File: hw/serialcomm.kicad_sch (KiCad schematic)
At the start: 4 parts, among them J2 USB_B_Micro, U17 W65C51NxP, U19 FT232RL, X4 1.8432 MHz

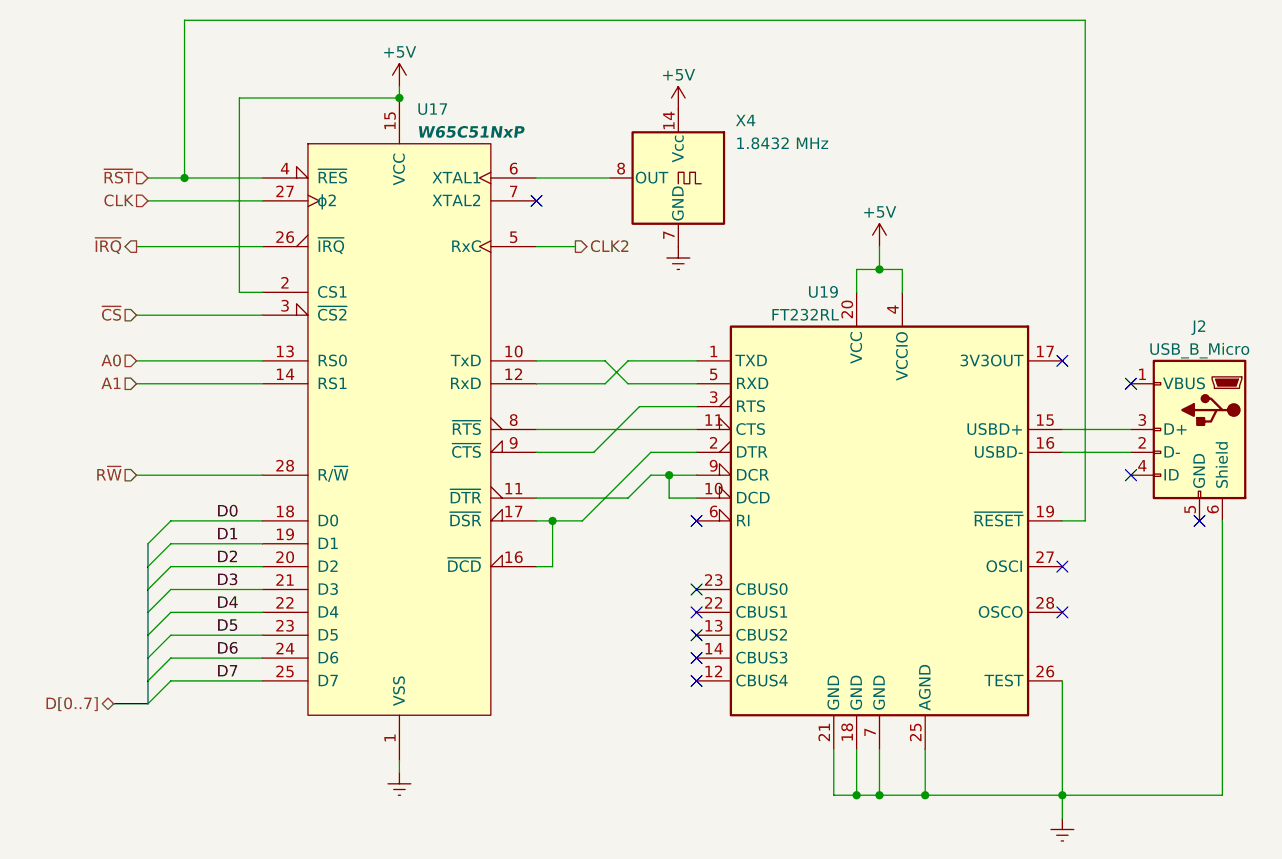
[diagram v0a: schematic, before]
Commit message: add hw design for veraduino
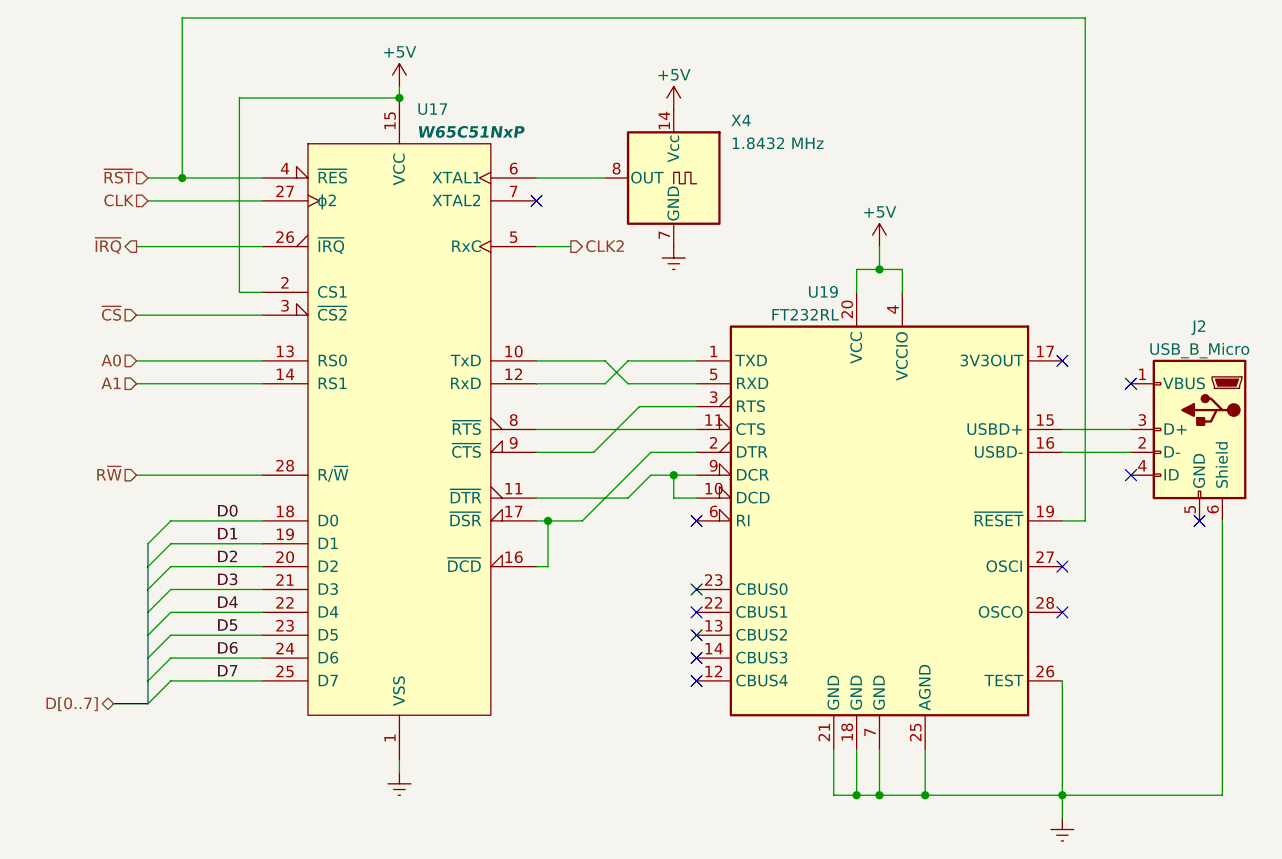
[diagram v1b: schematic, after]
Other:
- moved on the sheet: X4
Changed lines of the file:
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@@
   (junction (at 119.38 106.68) (diameter 0) (color 0 0 0 0)
   )
-  (junction (at 77.978 76.2) (diameter 0) (color 0 0 0 0)
-  )
-  (junction (at 90.932 71.12) (diameter 0) (color 0 0 0 0)
+  (junction (at 77.47 76.2) (diameter 0) (color 0 0 0 0)
+  )
+  (junction (at 91.44 71.12) (diameter 0) (color 0 0 0 0)
   )
   (junction (at 134.62 106.68) (diameter 0) (color 0 0 0 0)
   )
-  (junction (at 37.084 38.1) (diameter 0) (color 0 0 0 0)
+  (junction (at 36.83 38.1) (diameter 0) (color 0 0 0 0)
   )
   (junction (at 114.3 106.68) (diameter 0) (color 0 0 0 0)
@@
     (stroke (width 0) (type default))
   )
-  (wire (pts (xy 37.084 38.1) (xy 33.02 38.1))
+  (wire (pts (xy 36.83 38.1) (xy 33.02 38.1))
     (stroke (width 0) (type default))
   )
@@
     (stroke (width 0) (type default))
   )
-  (wire (pts (xy 88.9 71.12) (xy 90.932 71.12))
+  (wire (pts (xy 88.9 71.12) (xy 91.44 71.12))
     (stroke (width 0) (type default))
   )
@@
     (stroke (width 0) (type default))
   )
-  (wire (pts (xy 93.98 73.66) (xy 90.932 73.66))
+  (wire (pts (xy 93.98 73.66) (xy 91.44 73.66))
     (stroke (width 0) (type default))
   )
@@
     (stroke (width 0) (type default))
   )
-  (wire (pts (xy 90.932 71.12) (xy 93.98 71.12))
+  (wire (pts (xy 91.44 71.12) (xy 93.98 71.12))
     (stroke (width 0) (type default))
   )
@@
     (stroke (width 0) (type default))
   )
-  (wire (pts (xy 45.72 38.1) (xy 37.084 38.1))
-    (stroke (width 0) (type default))
-  )
-  (wire (pts (xy 76.2 45.72) (xy 80.518 45.72))
+  (wire (pts (xy 45.72 38.1) (xy 36.83 38.1))
+    (stroke (width 0) (type default))
+  )
+  (wire (pts (xy 76.2 45.72) (xy 80.01 45.72))
     (stroke (width 0) (type default))
   )
@@
     (stroke (width 0) (type default))
   )
-  (wire (pts (xy 137.16 20.574) (xy 37.084 20.574))
+  (wire (pts (xy 137.16 20.32) (xy 36.83 20.32))
     (stroke (width 0) (type default))
   )
@@
     (stroke (width 0) (type default))
   )
-  (wire (pts (xy 76.2 38.1) (xy 84.328 38.1))
+  (wire (pts (xy 76.2 38.1) (xy 83.82 38.1))
     (stroke (width 0) (type default))
   )
@@
     (stroke (width 0) (type default))
   )
-  (wire (pts (xy 37.084 20.574) (xy 37.084 38.1))
-    (stroke (width 0) (type default))
-  )
-  (wire (pts (xy 90.932 73.66) (xy 90.932 71.12))
+  (wire (pts (xy 36.83 20.32) (xy 36.83 38.1))
+    (stroke (width 0) (type default))
+  )
+  (wire (pts (xy 91.44 73.66) (xy 91.44 71.12))
     (stroke (width 0) (type default))
   )
@@
     (stroke (width 0) (type default))
   )
-  (wire (pts (xy 77.978 81.28) (xy 77.978 76.2))
-    (stroke (width 0) (type default))
-  )
-  (wire (pts (xy 77.978 76.2) (xy 81.28 76.2))
+  (wire (pts (xy 77.47 81.28) (xy 77.47 76.2))
+    (stroke (width 0) (type default))
+  )
+  (wire (pts (xy 77.47 76.2) (xy 81.28 76.2))
     (stroke (width 0) (type default))
   )
@@
     (stroke (width 0) (type default))
   )
-  (wire (pts (xy 76.2 81.28) (xy 77.978 81.28))
+  (wire (pts (xy 76.2 81.28) (xy 77.47 81.28))
     (stroke (width 0) (type default))
   )
@@
     (stroke (width 0) (type default))
   )
-  (wire (pts (xy 137.16 20.574) (xy 137.16 76.2))
-    (stroke (width 0) (type default))
-  )
-  (wire (pts (xy 76.2 76.2) (xy 77.978 76.2))
+  (wire (pts (xy 137.16 20.32) (xy 137.16 76.2))
+    (stroke (width 0) (type default))
+  )
+  (wire (pts (xy 76.2 76.2) (xy 77.47 76.2))
     (stroke (width 0) (type default))
   )
@@
     (effects (font (size 1.27 1.27)) (justify right))
   )
-  (hierarchical_label "CLK2" (shape output) (at 80.518 45.72 0) (fields_autoplaced)
+  (hierarchical_label "CLK2" (shape output) (at 80.01 45.72 0) (fields_autoplaced)
     (effects (font (size 1.27 1.27)) (justify left))
   )
@@
     )
   )
-  (symbol (lib_id "power:VCC") (at 91.948 30.48 0) (unit 1)
+  (symbol (lib_id "power:VCC") (at 91.44 30.48 0) (unit 1)
     (in_bom yes) (on_board yes) (dnp no) (fields_autoplaced)
-    (property "Reference" "#PWR025" (at 91.948 34.29 0)
-      (effects (font (size 1.27 1.27)) hide)
-    )
-    (property "Value" "+5V" (at 91.948 26.67 0)
+    (property "Reference" "#PWR025" (at 91.44 34.29 0)
+      (effects (font (size 1.27 1.27)) hide)
+    )
+    (property "Value" "+5V" (at 91.44 26.67 0)
       (effects (font (size 1.27 1.27)))
     )
-    (property "Footprint" "" (at 91.948 30.48 0)
-      (effects (font (size 1.27 1.27)) hide)
-    )
-    (property "Datasheet" "" (at 91.948 30.48 0)
+    (property "Footprint" "" (at 91.44 30.48 0)
+      (effects (font (size 1.27 1.27)) hide)
+    )
+    (property "Datasheet" "" (at 91.44 30.48 0)
       (effects (font (size 1.27 1.27)) hide)
     )
@@
     )
   )
-  (symbol (lib_id "power:Earth") (at 91.948 45.72 0) (unit 1)
+  (symbol (lib_id "power:Earth") (at 91.44 45.72 0) (unit 1)
     (in_bom yes) (on_board yes) (dnp no) (fields_autoplaced)
-    (property "Reference" "#PWR026" (at 91.948 52.07 0)
-      (effects (font (size 1.27 1.27)) hide)
-    )
-    (property "Value" "Earth" (at 91.948 49.53 0)
-      (effects (font (size 1.27 1.27)) hide)
-    )
-    (property "Footprint" "" (at 91.948 45.72 0)
-      (effects (font (size 1.27 1.27)) hide)
-    )
-    (property "Datasheet" "~" (at 91.948 45.72 0)
+    (property "Reference" "#PWR026" (at 91.44 52.07 0)
+      (effects (font (size 1.27 1.27)) hide)
+    )
+    (property "Value" "Earth" (at 91.44 49.53 0)
+      (effects (font (size 1.27 1.27)) hide)
+    )
+    (property "Footprint" "" (at 91.44 45.72 0)
+      (effects (font (size 1.27 1.27)) hide)
+    )
+    (property "Datasheet" "~" (at 91.44 45.72 0)
       (effects (font (size 1.27 1.27)) hide)
     )
@@
     )
   )
-  (symbol (lib_id "Oscillator:ACO-xxxMHz") (at 91.948 38.1 0) (mirror y) (unit 1)
+  (symbol (lib_id "Oscillator:ACO-xxxMHz") (at 91.44 38.1 0) (mirror y) (unit 1)
     (in_bom yes) (on_board yes) (dnp no)
-    (property "Reference" "X4" (at 98.298 31.75 0)
+    (property "Reference" "X4" (at 97.79 31.75 0)
       (effects (font (size 1.27 1.27)) (justify right))
     )
-    (property "Value" "1.8432 MHz" (at 98.298 34.29 0)
+    (property "Value" "1.8432 MHz" (at 97.79 34.29 0)
       (effects (font (size 1.27 1.27)) (justify right))
     )
-    (property "Footprint" "Oscillator:Oscillator_DIP-14" (at 80.518 46.99 0)
-      (effects (font (size 1.27 1.27)) hide)
-    )
-    (property "Datasheet" "http://www.conwin.com/datasheets/cx/cx030.pdf" (at 94.488 38.1 0)
-      (effects (font (size 1.27 1.27)) hide)
-    )
+    (property "Footprint" "Oscillator:Oscillator_DIP-14" (at 80.01 46.99 0)
+      (effects (font (size 1.27 1.27)) hide)
+    )
+    (property "Datasheet" "http://www.conwin.com/datasheets/cx/cx030.pdf" (at 93.98 38.1 0)
+      (effects (font (size 1.27 1.27)) hide)
+    )
